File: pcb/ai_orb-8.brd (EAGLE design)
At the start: 44.5 x 44.5 mm, 30 parts

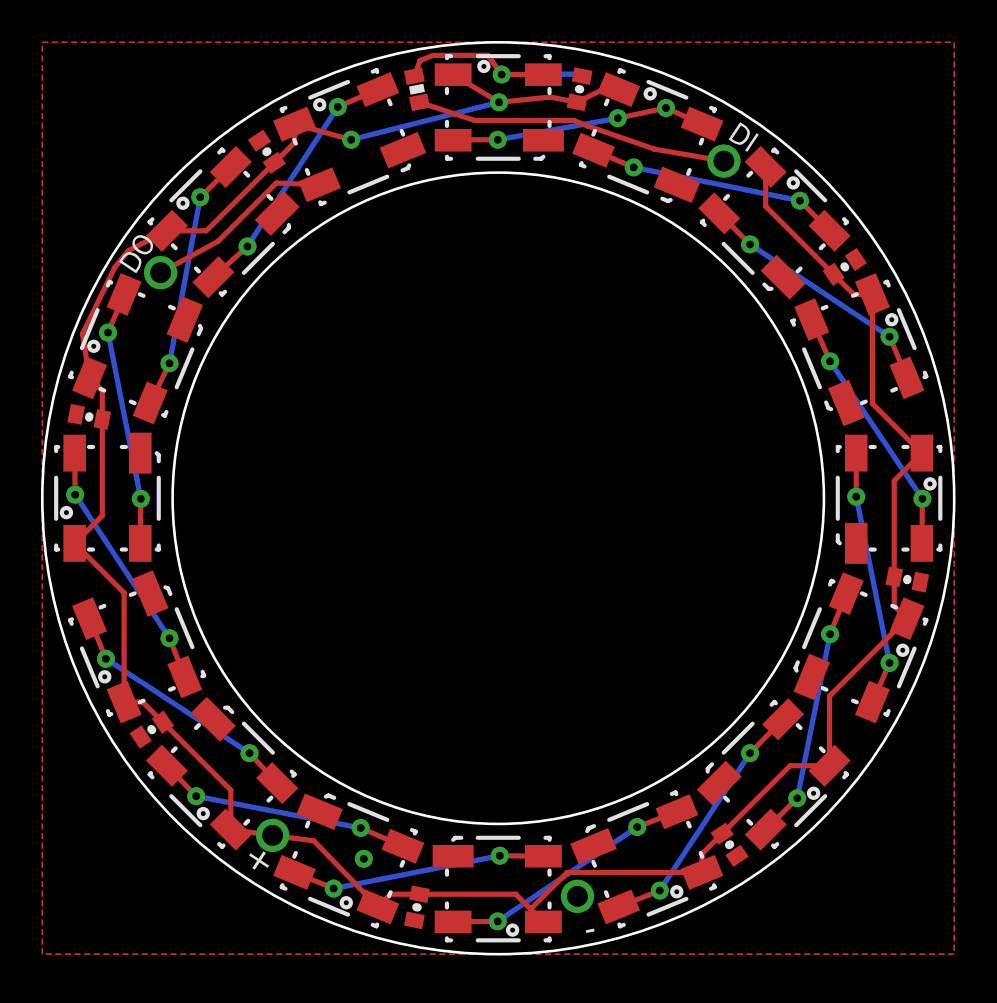
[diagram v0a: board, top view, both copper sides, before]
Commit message: updating
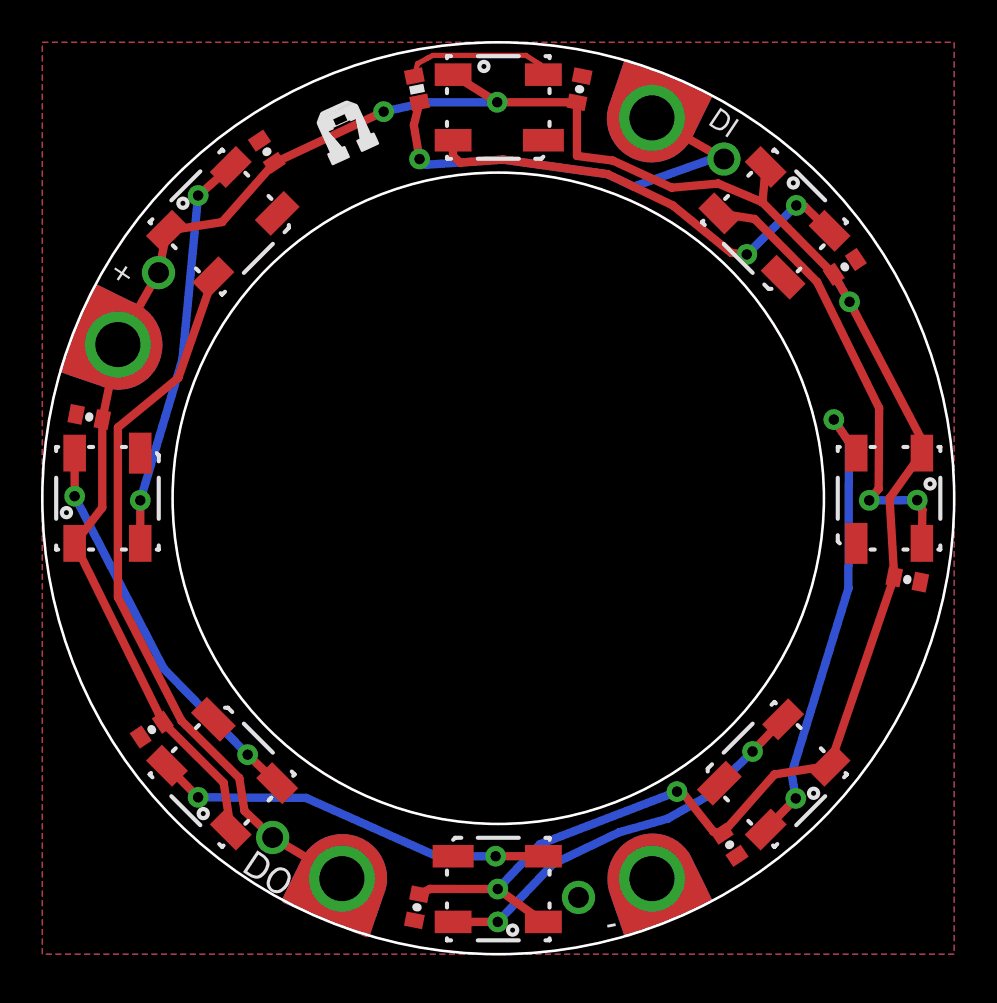
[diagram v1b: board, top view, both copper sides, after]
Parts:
- removed LED10, LED12, LED14, LED16, LED2, LED4, LED6, LED8: LED-WS2812B-SM, Ai_LED:LED-WS2812B-SM
- added +', -', DI', DO': 1X01-PETAL, Ai_Connectors:1X01-PETAL
- added LOGO1: AI-LOGOXS, Ai_Miscellany:AI-LOGO-XS
- moved DO 28.1 mm to (11.2, 5.69)
- moved + 28.0 mm to (5.66, 33.2)
- moved DI 0.10 mm to (33.2, 38.8)
- moved - 0.07 mm to (26.1, 2.77)
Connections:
- removed net N$11: LED10.2, LED11.4
- removed net N$12: LED11.2, LED12.4
- removed net N$15: LED14.2, LED15.4
- removed net N$16: LED15.2, LED16.4
- removed net N$3: DI.1, R1.2
- removed net N$5: LED4.2, LED5.4
- removed net N$7: LED6.2, LED7.4
- removed net N$8: LED7.2, LED8.4
- net DO: now also DO'.1, LED15.2; no longer LED16.2
- net GND: now also -'.1; no longer LED10.3, LED12.3, LED14.3, LED16.3, LED2.3, LED4.3, LED6.3, LED8.3
- net N$1: now also LED3.4; no longer LED2.4
- net N$10: now also LED11.4; no longer LED10.4
- net N$13: now also LED11.2; no longer LED12.2
- net N$14: now also LED15.4; no longer LED14.4
- net N$2: now also DI'.1, DI.1, R1.2; no longer LED2.2, LED3.4
- net N$4: now also LED5.4; no longer LED4.4
- net N$6: now also LED7.4; no longer LED6.4
- net N$9: now also LED7.2; no longer LED8.2
- net VCC: now also +'.1; no longer LED10.1, LED12.1, LED14.1, LED16.1, LED2.1, LED4.1, LED6.1, LED8.1
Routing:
- net DO: track 9.32 -> 35.5 mm
- net N$3: track 15.3 -> 0.00 mm
- net N$8: track 12.5 -> 0.00 mm, vias 2 -> 0
- net N$15: track 12.5 -> 0.00 mm, vias 2 -> 0
- net N$12: track 12.5 -> 0.00 mm, vias 2 -> 0
- net N$11: track 12.5 -> 0.00 mm, vias 2 -> 0
- net N$16: track 12.5 -> 0.00 mm, vias 2 -> 0
- net N$5: track 12.5 -> 0.00 mm, vias 2 -> 0
- net N$7: track 12.5 -> 0.00 mm, vias 2 -> 0
- net N$6: track 12.5 -> 23.2 mm
- net N$2: track 12.5 -> 22.2 mm, vias 2 -> 1
- net N$4: track 12.5 -> 22.1 mm
- net N$1: track 12.5 -> 22.0 mm, vias 3 -> 2
- net N$10: track 12.4 -> 19.6 mm
- net N$9: track 12.5 -> 19.6 mm
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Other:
- board text added: "ORB-8"
- board text removed: "ORB-16"
